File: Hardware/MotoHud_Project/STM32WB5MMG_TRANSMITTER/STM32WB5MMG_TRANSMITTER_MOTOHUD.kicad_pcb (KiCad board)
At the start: 2 copper layers, 46 x 77 mm, 4 parts, among them J1 MCP2515_CAN, J3 12V_RAIL

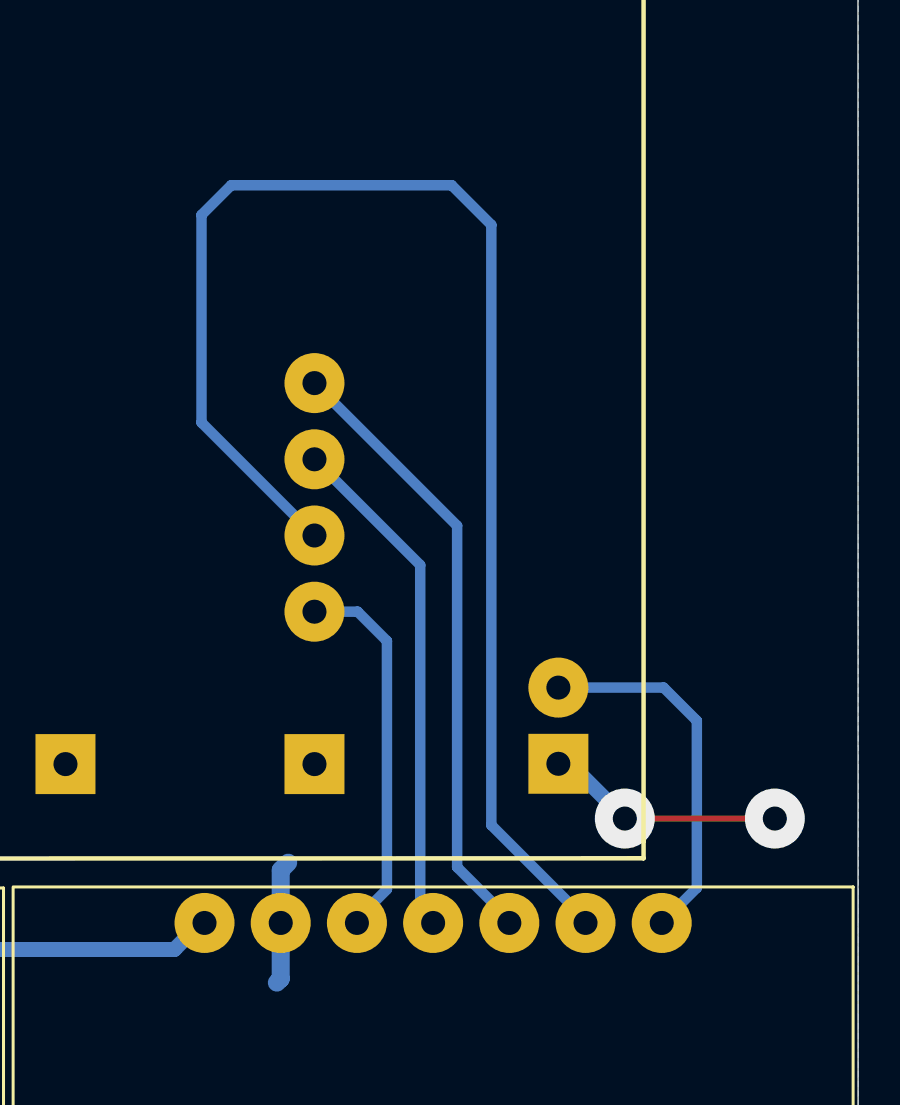
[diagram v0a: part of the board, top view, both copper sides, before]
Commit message: updated hardware
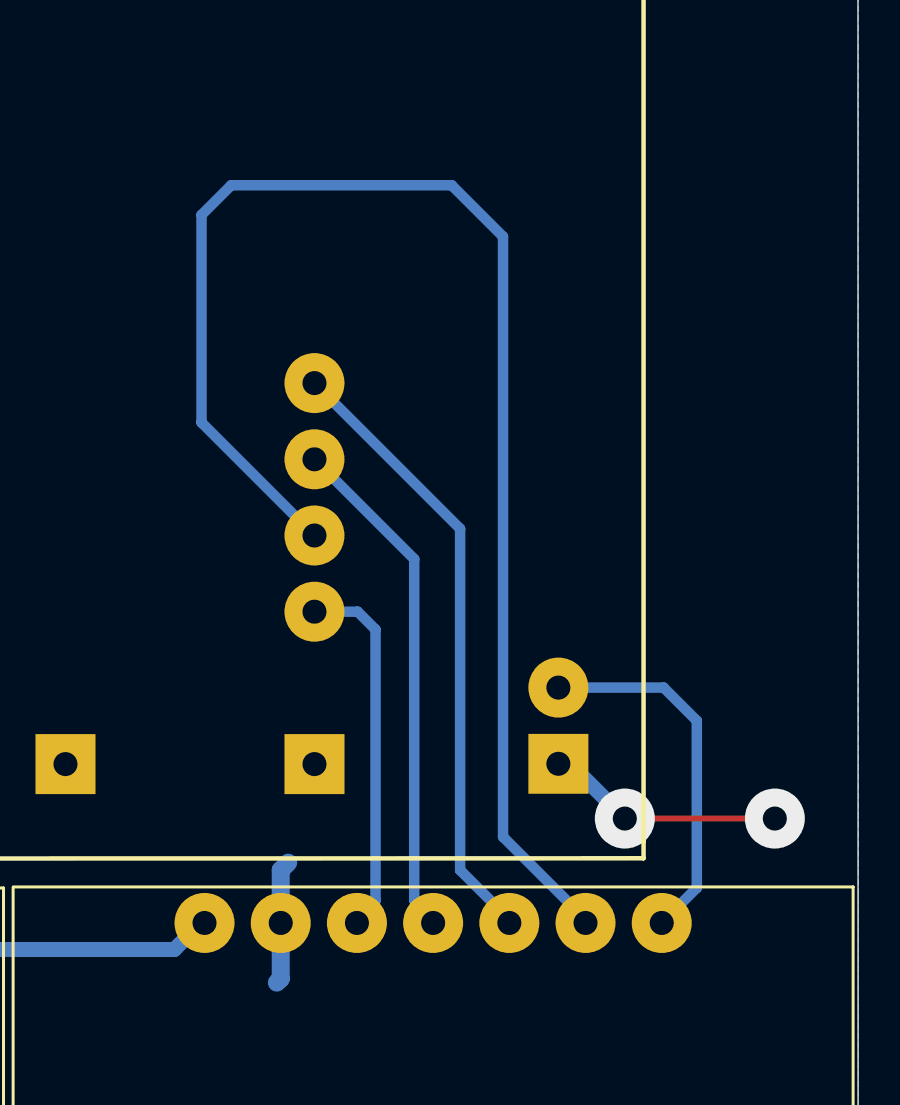
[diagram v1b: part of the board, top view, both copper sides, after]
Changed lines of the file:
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@@
+	(segment
+		(start 138.655 94.105)
+		(end 138.65 94.11)
+		(width 0.35)
+		(layer "B.Cu")
+		(net 4)
+	)
+	(segment
+		(start 140.69 103.74)
+		(end 140.07 104.36)
+		(width 0.35)
+		(layer "B.Cu")
+		(net 4)
+	)
+	(segment
+		(start 140.095 94.105)
+		(end 140.69 94.7)
+		(width 0.35)
+		(layer "B.Cu")
+		(net 4)
+	)
+	(segment
+		(start 140.69 94.7)
+		(end 140.69 103.74)
+		(width 0.35)
+		(layer "B.Cu")
+		(net 4)
+	)
 	(segment
 		(start 138.655 94.105)
@@
 	)
 	(segment
-		(start 141.07 103.36)
-		(end 140.07 104.36)
+		(start 143.51 102.72)
+		(end 145.15 104.36)
 		(width 0.35)
 		(layer "B.Cu")
-		(net 4)
+		(net 5)
 	)
 	(segment
-		(start 138.655 94.105)
-		(end 138.65 94.11)
-		(width 0.35)
-		(layer "B.Cu")
-		(net 4)
-	)
-	(segment
-		(start 140.095 94.105)
-		(end 141.07 95.08)
-		(width 0.35)
-		(layer "B.Cu")
-		(net 4)
-	)
-	(segment
-		(start 141.07 95.08)
-		(end 141.07 103.36)
-		(width 0.35)
-		(layer "B.Cu")
-		(net 4)
-	)
-	(segment
-		(start 143.41 91.24)
-		(end 143.41 102.62)
+		(start 143.51 91.34)
+		(end 143.51 102.72)
 		(width 0.35)
 		(layer "B.Cu")
@@
 	(segment
 		(start 138.655 86.485)
-		(end 143.41 91.24)
+		(end 143.51 91.34)
 		(width 0.35)
 		(layer "B.Cu")
@@
 	)
 	(segment
-		(start 143.41 102.62)
-		(end 145.15 104.36)
-		(width 0.35)
-		(layer "B.Cu")
-		(net 5)
-	)
-	(segment
-		(start 142.18 92.55)
-		(end 142.18 103.93)
+		(start 141.98 92.35)
+		(end 141.98 103.73)
 		(width 0.35)
 		(layer "B.Cu")
@@
 	)
 	(segment
-		(start 142.18 103.93)
+		(start 138.655 89.025)
+		(end 141.98 92.35)
+		(width 0.35)
+		(layer "B.Cu")
+		(net 6)
+	)
+	(segment
+		(start 141.98 103.73)
 		(end 142.61 104.36)
 		(width 0.35)
@@
 	)
 	(segment
-		(start 138.655 89.025)
-		(end 142.18 92.55)
-		(width 0.35)
-		(layer "B.Cu")
-		(net 6)
-	)
-	(segment
-		(start 134.89 80.88)
-		(end 135.88 79.89)
+		(start 143.23 79.89)
+		(end 144.94 81.6)
 		(width 0.35)
 		(layer "B.Cu")
@@
 	)
 	(segment
-		(start 143.23 79.89)
-		(end 144.55 81.21)
+		(start 144.94 81.6)
+		(end 144.94 101.61)
 		(width 0.35)
 		(layer "B.Cu")
@@
 	)
 	(segment
-		(start 144.55 101.22)
-		(end 147.69 104.36)
-		(width 0.35)
-		(layer "B.Cu")
-		(net 7)
-	)
-	(segment
-		(start 144.55 81.21)
-		(end 144.55 101.22)
+		(start 134.89 80.88)
+		(end 135.88 79.89)
 		(width 0.35)
 		(layer "B.Cu")
@@
 		(width 0.35)
 		(layer "B.Cu")
+		(net 7)
+	)
+	(segment
+		(start 144.94 101.61)
+		(end 147.69 104.36)
+		(width 0.35)
+		(layer "B.Cu")
